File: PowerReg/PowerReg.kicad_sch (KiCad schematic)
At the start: 6 parts, among them U2 TPS62172DSG

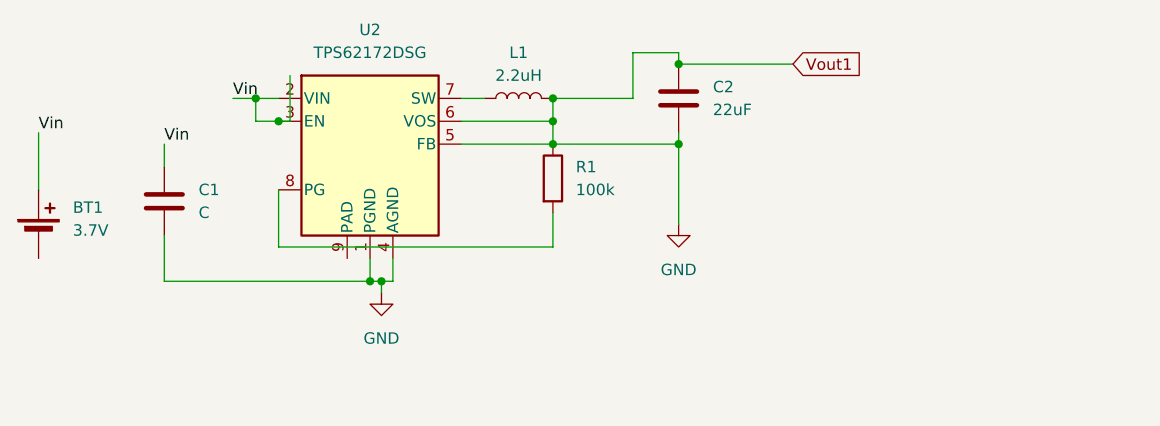
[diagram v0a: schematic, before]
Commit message: Add files via upload
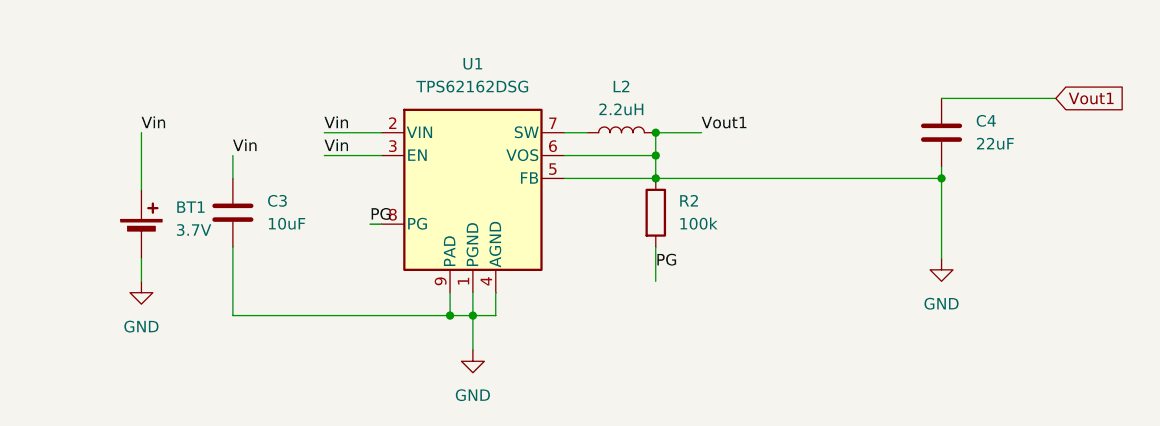
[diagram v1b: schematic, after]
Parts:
- removed C1: C, symbol Device:C
- removed C2: 22uF, symbol Device:C
- removed L1: 2.2uH, symbol Device:L
- removed R1: 100k, symbol Device:R
- removed U2: TPS62172DSG, Package_SON:WSON-8-1EP_2x2mm_P0.5mm_EP0.9x1.6mm_ThermalVias, symbol Regulator_Switching:TPS62172DSG
- added C3: 10uF, symbol Device:C
- added C4: 22uF, symbol Device:C
- added L2: 2.2uH, symbol Device:L
- added R2: 100k, symbol Device:R
- added U1: TPS62162DSG, Package_SON:WSON-8-1EP_2x2mm_P0.5mm_EP0.9x1.6mm_ThermalVias, symbol Regulator_Switching:TPS62162DSG
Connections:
- net GND: now also BT1.2 (-), C3.2, C4.1, C4.2, L2.2, R2.1, U1.1 (PGND), U1.4 (AGND), U1.5 (FB), U1.6 (VOS), U1.9 (PAD)
- net Vin: now also C3.1, U1.2 (VIN), U1.3 (EN)
- new net: L2.1, U1.7 (SW)
- new net PG: R2.2, U1.8 (PG)
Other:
- moved on the sheet: BT1
